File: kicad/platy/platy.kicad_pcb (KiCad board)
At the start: 2 copper layers, 100 x 100 mm, 90 parts, among them J1 Conn_01x04_Socket, J2 Conn_01x02_Socket, J5 USB_C_Receptacle_USB2.0_16P, J6 Conn_01x04_Pin, J8 Conn_01x14_Socket, J9 Conn_02x04_Odd_Even, Q4 BC847, Q5 Q_PMOS_GSD, SW1 SW_DPST, SW2 SW_Push(Boot), SW3 SW_Push(EN), U10 ESP32-S3-WROOM-1, U4 CC1101, U5 PN5321A3HN_C1xx, U6 TSOP382xx, U7 AMS1117-3.3, Y2 27.12Mhz, Y3 26MHz

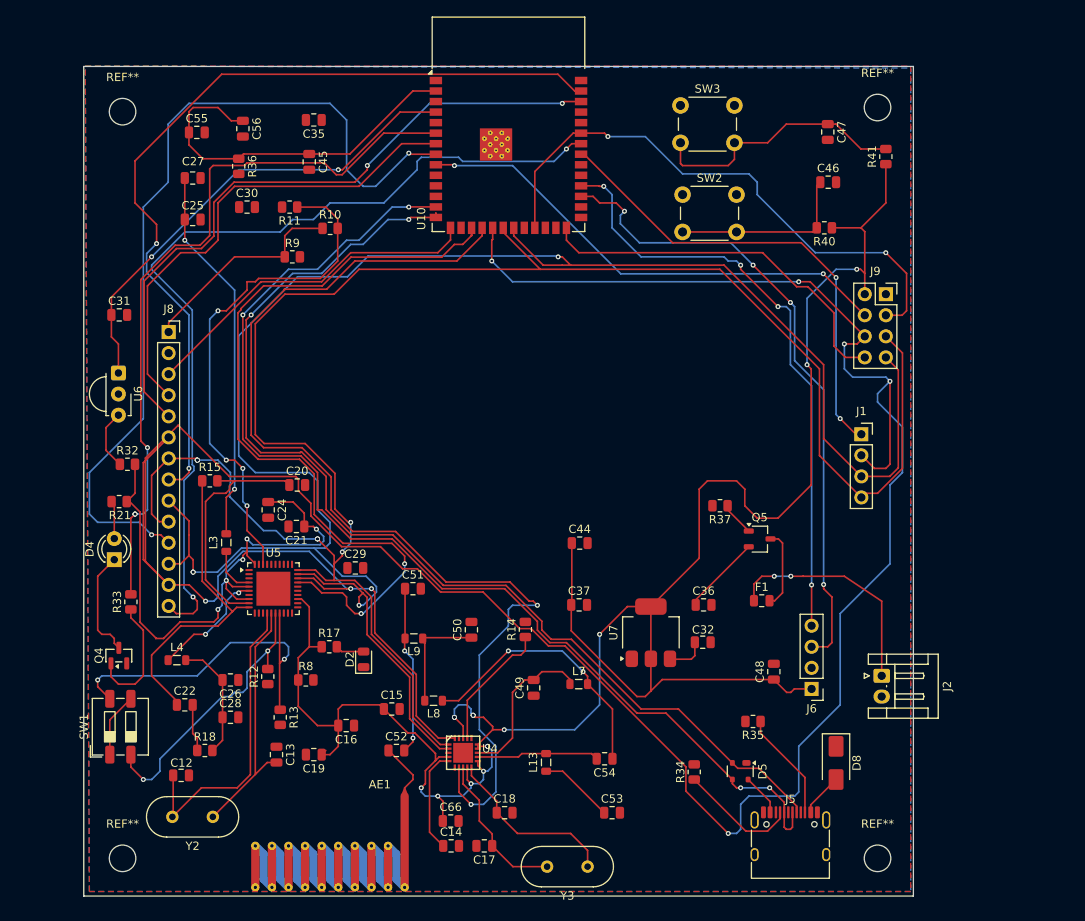
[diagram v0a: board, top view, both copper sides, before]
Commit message: made the second ertation of the pcb
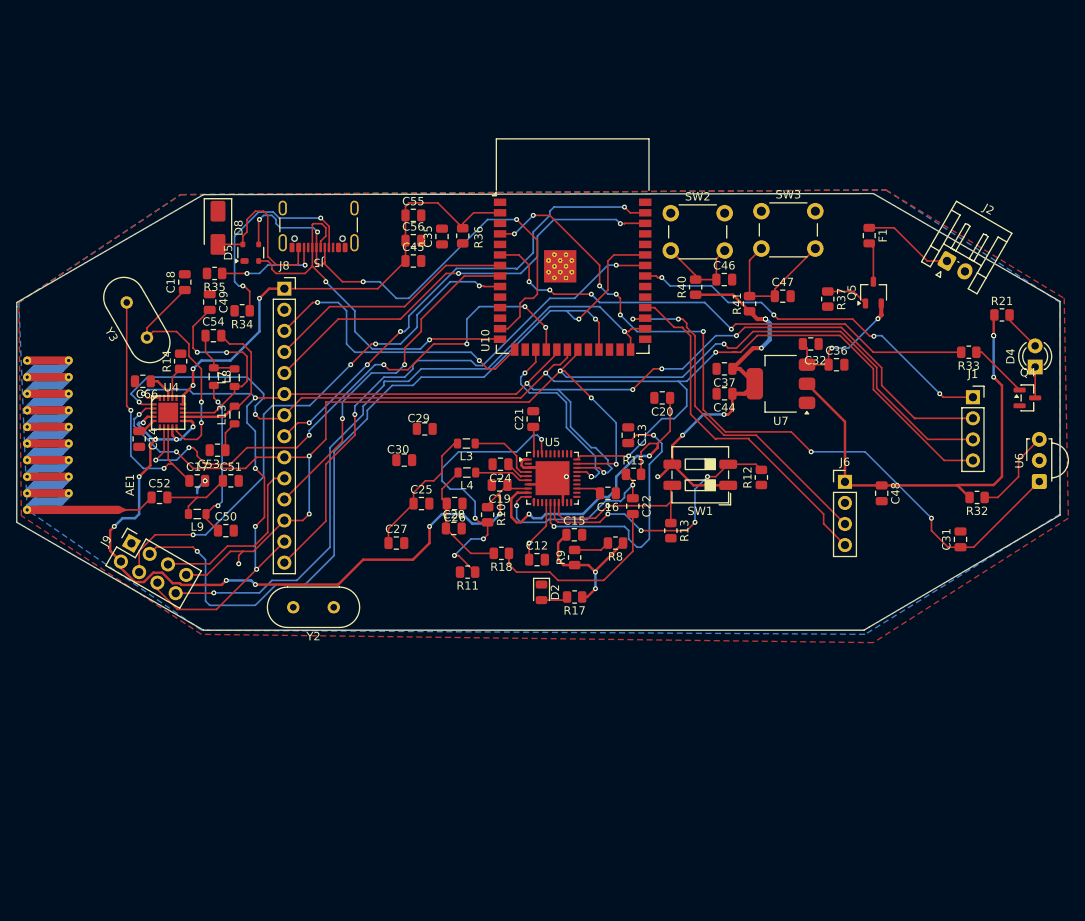
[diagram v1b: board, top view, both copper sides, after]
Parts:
- removed REF** (x4): MountingHole_3.2mm_M3, MountingHole:MountingHole_3.2mm_M3
- J5: footprint Connector_USB:USB_C_Receptacle_HRO_TYPE-C-31-M-12 -> Connector_USB:USB_C_Receptacle_GCT_USB4105-xx-A_16P_TopMnt_Horizontal
- moved Q4 113.8 mm to (216.6, 89.5), turned to 0 degrees
- moved D4 113.4 mm to (217.5, 85.8)
- moved U6 111.8 mm to (218.0, 99.6), turned to 90 degrees
- moved R21 108.8 mm to (213.5, 79.5), turned to 0 degrees
- moved R33 105.4 mm to (209.5, 84.0), turned to 180 degrees
- moved C31 104.9 mm to (208.5, 106.5), turned to 90 degrees
- moved R32 102.5 mm to (210.5, 101.5), turned to 180 degrees
- moved D8 98.5 mm to (119.0, 69.0)
- moved J9 95.8 mm to (108.6, 107.0), turned to 60 degrees
- moved J5 94.8 mm to (131.1, 67.7), turned to 180 degrees
- moved D5 85.9 mm to (123.0, 72.0), turned to 90 degrees
- moved R35 84.4 mm to (118.6, 74.5)
- moved Y3 83.0 mm to (110.4, 82.2), turned to 120 degrees
- moved R34 77.8 mm to (121.9, 79.0), turned to 180 degrees
- moved SW1 76.2 mm to (177.1, 98.8), turned to 180 degrees
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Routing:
- net /MOSI: track 341.7 -> 178.6 mm, vias 8 -> 10
- net /3v3: track 411.0 -> 287.8 mm, vias 19 -> 24
- net /USB_D+: track 131.3 -> 46.4 mm
- net /SSEL: track 97.1 -> 24.5 mm, vias 2 -> 3
- net /USB_D-: track 136.6 -> 64.1 mm
- net /SCK: track 232.6 -> 169.3 mm, vias 7 -> 5
- net /CSN: track 104.6 -> 42.0 mm
- net /CSn: track 128.7 -> 67.3 mm, vias 2 -> 7
- net /MISO: track 234.3 -> 173.3 mm, vias 4 -> 9
- net /led: track 103.0 -> 57.9 mm, vias 2 -> 4
- net /irq_tht: track 107.6 -> 65.2 mm
- net /GPIO 4: track 57.9 -> 94.8 mm, vias 2 -> 8
- net /IRQ: track 45.7 -> 82.6 mm, vias 0 -> 2
- net /Vrx: track 77.8 -> 42.6 mm, vias 4 -> 2
- net /CE: track 68.6 -> 101.9 mm, vias 2 -> 3
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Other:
- board size 100 x 100 mm -> 125.8 x 52.6 mm
